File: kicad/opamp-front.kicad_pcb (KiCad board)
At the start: 2 copper layers, 101.3 x 102.4 mm, 91 parts, among them J1 INPUT, J2 GND, J3 SPK, J4 GND, J5 B+, J6 B-, Q1 BD140, Q10 BD139, Q11 BD139, Q12 BD140, Q13 MJL1302C, Q2 2N3906, Q3 2N5551, Q4 2N5401, Q5 2N5551, Q6 2N5401, Q7 BD139, Q8 2N3904, Q9 MJL3281C, U1 LM4562

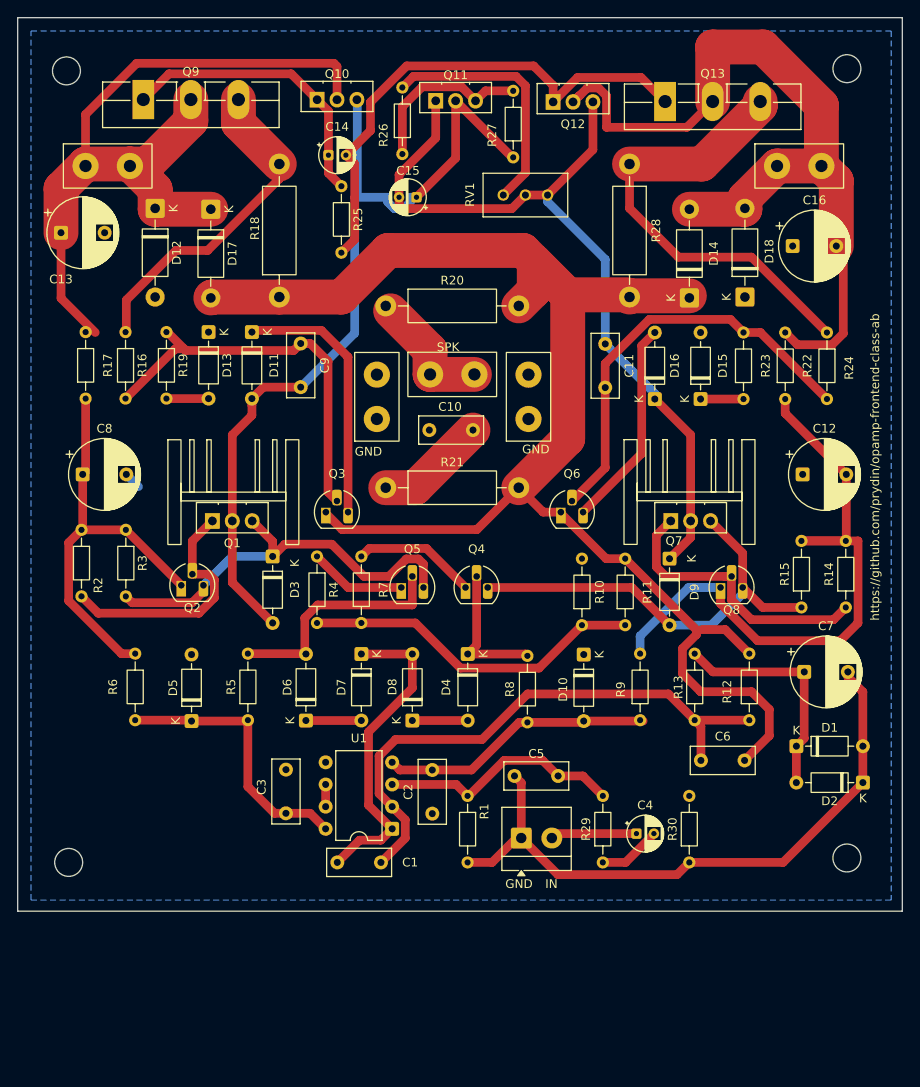
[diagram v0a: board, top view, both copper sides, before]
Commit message: WIP
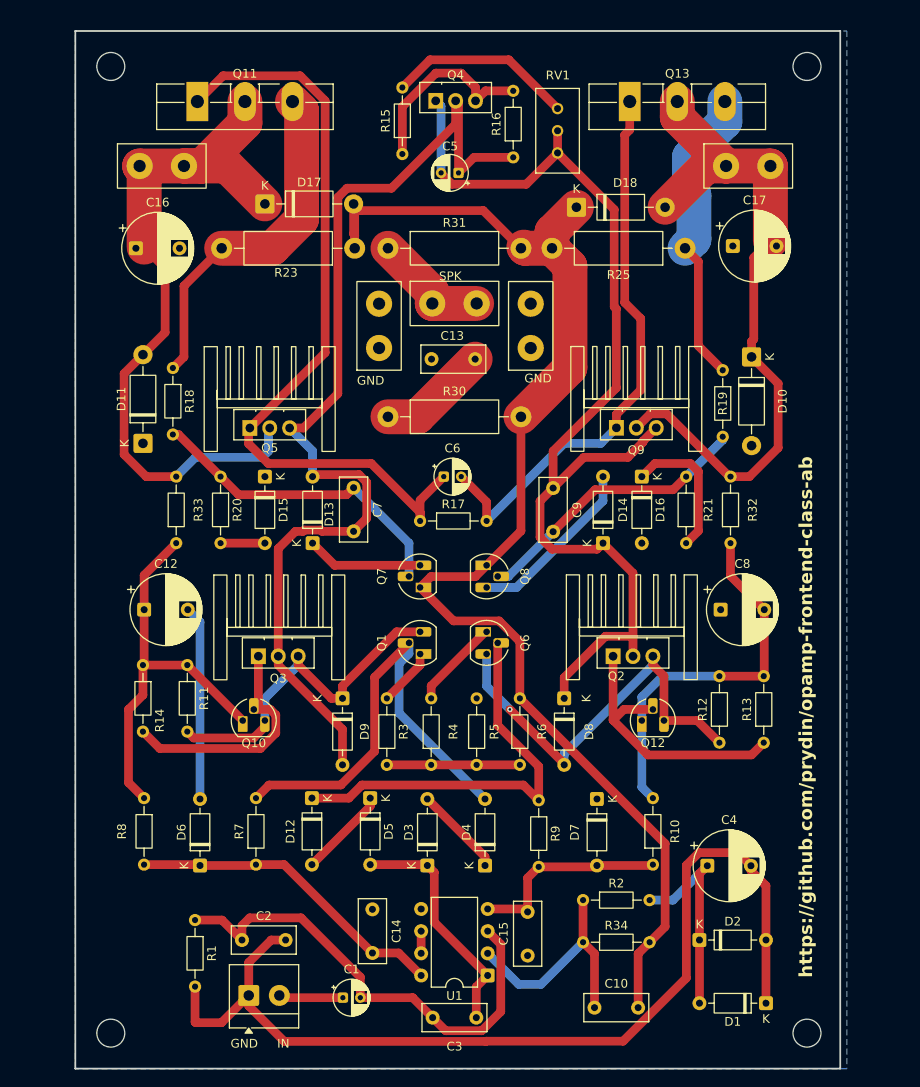
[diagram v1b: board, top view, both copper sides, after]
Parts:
- removed the Q10 at (85.1, 41.9)
- removed R29: 470, Resistor_THT:R_Axial_DIN0204_L3.6mm_D1.6mm_P7.62mm_Horizontal
- removed the R30 at (127.7, 129.3)
- added Q5: BD139, Package_TO_SOT_THT:TO-126-3_Vertical, F.Cu at (77.4, 79.5)
- added REF**: Heatsink, Custom:Heatsink, F.Cu at (79.7, 75.2)
- added REF**: Heatsink, Custom:Heatsink, F.Cu at (121.7, 75.2)
- Q10: renamed from Q2; value 2N3906 -> 2N2906
- Q12: renamed from Q8; value 2N3904 -> 2N2904
- moved C2 40.8 mm to (76.5, 138.2), turned to 0 degrees
- moved R17 39.4 mm to (96.9, 90.2), turned to 0 degrees
- moved C6 39.1 mm to (99.6, 85.1)
- moved C1 38.5 mm to (88.1, 144.8)
- moved Q9 38.0 mm to (119.4, 79.5)
- moved J3 36.1 mm to (77.3, 144.5)
- moved R1 34.3 mm to (71.1, 135.9)
- moved R34 31.8 mm to (115.6, 138.4), turned to 0 degrees
- moved C10 30.8 mm to (116.9, 145.9)
- moved D1 27.6 mm to (136.5, 145.4)
- moved D11 27.0 mm to (65.2, 81.3), turned to 90 degrees
- moved D4 26.4 mm to (104.3, 129.6)
- moved D3 25.4 mm to (97.7, 129.6), turned to 90 degrees
- moved D13 25.2 mm to (84.6, 92.7), turned to 90 degrees
- moved C4 24.8 mm to (129.8, 129.7)
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- renumbered C4 to C1, C6 to C10, C8 to C12, C10 to C13, C3 to C14, C2 to C15, C13 to C16, C16 to C17, C5 to C2, C1 to C3, C7 to C4, C15 to C5, C14 to C6, C9 to C7, C12 to C8, C11 to C9, D2 to D1, D18 to D10, D12 to D11, D4 to D12, D11 to D13, D16 to D14, D13 to D15, D15 to D16, D14 to D18, D1 to D2, D7 to D3, D6 to D4, D8 to D5, D5 to D6, D10 to D7, D9 to D8, D3 to D9, J5 to J1, J3 to J2, J1 to J3, J6 to J5, J2 to J6, Q5 to Q1, Q9 to Q11, Q7 to Q2, Q1 to Q3, Q11 to Q4, Q4 to Q6, Q3 to Q7, Q6 to Q8, Q12 to Q9, R9 to R10, R3 to R11, R15 to R12, R14 to R13, R2 to R14, R26 to R15, R27 to R16, R25 to R17, R16 to R18, R24 to R19, R13 to R2, R19 to R20, R23 to R21, R18 to R23, R28 to R25, R4 to R3, R21 to R30, R20 to R31, R22 to R32, R17 to R33, R12 to R34, R7 to R4, R10 to R5, R11 to R6, R5 to R7, R6 to R8, R8 to R9
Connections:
- C1 pad 2: Net-(C4-Pad2) -> Net-(U1A-+)
- C3 pad 1: Net-(U1A--) -> Net-(U1A-+)
- D10 pad 1: GND -> /B-
- D10 pad 2: /B- -> GND
- D11 pad 1: /B+ -> GND
- D11 pad 2: GND -> /B+
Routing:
- net Net-(Q11-B): track 33.4 -> 90.1 mm
- net GNDA: track 72.8 -> 114.6 mm
- net Net-(U1A--): track 66.1 -> 27.3 mm
- net Net-(D14-K): track 93.8 -> 126.2 mm
- net Net-(D12-K): track 16.2 -> 47.3 mm
- net Net-(Q12-E): track 73.8 -> 43.8 mm
- net Net-(U1A-+): track 27.9 -> 55.5 mm
- net Net-(D4-A): track 27.1 -> 52.3 mm
- net Net-(R3-Pad2): track 39.5 -> 15.2 mm
- net Net-(D17-A): track 177.5 -> 154.4 mm
- net Net-(D13-A): track 101.1 -> 121.6 mm
- net GND: track 1.98 -> 22.3 mm
- net /B-: track 96.2 -> 78.3 mm
- net Net-(Q13-E): track 51.8 -> 34.9 mm
- net Net-(D13-K): track 29.8 -> 13.4 mm
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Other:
- board size 101.3 x 102.4 mm -> 87.6 x 118.9 mm

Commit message: Restored after rebase mishap
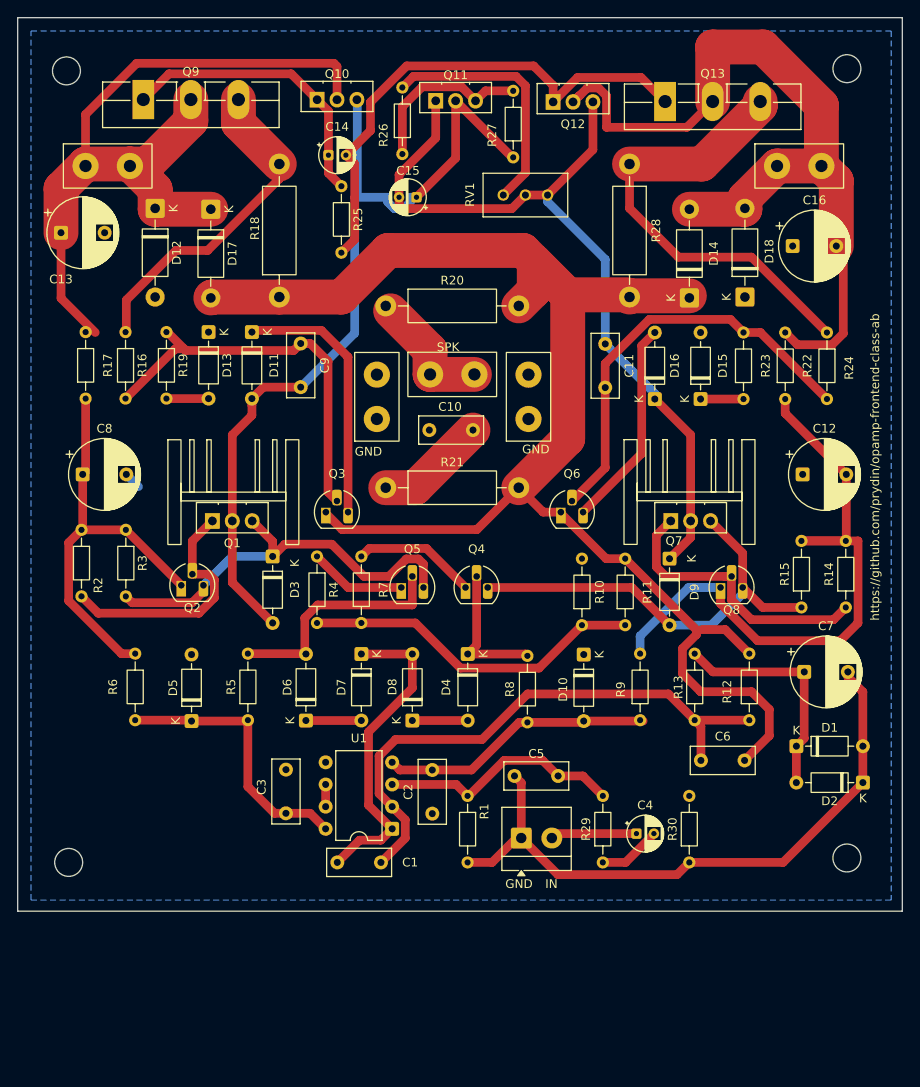
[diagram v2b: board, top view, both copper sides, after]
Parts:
- removed the Q5 at (77.4, 79.5)
- removed the REF** at (79.7, 75.2)
- removed the REF** at (121.7, 75.2)
- added Q10: BD139, Package_TO_SOT_THT:TO-126-3_Vertical, F.Cu at (85.1, 41.9)
- added R29: 470, Resistor_THT:R_Axial_DIN0204_L3.6mm_D1.6mm_P7.62mm_Horizontal, F.Cu at (117.8, 129.3)
- added R30: 10, Resistor_THT:R_Axial_DIN0204_L3.6mm_D1.6mm_P7.62mm_Horizontal, F.Cu at (127.7, 129.3)
- Q2: renamed from Q10; value 2N2906 -> 2N3906
- Q8: renamed from Q12; value 2N2904 -> 2N3904
- moved C5 40.8 mm to (112.7, 119.4), turned to 180 degrees
- moved R25 39.4 mm to (87.9, 51.8), turned to -90 degrees
- moved C14 39.1 mm to (86.4, 48.3)
- moved C4 38.5 mm to (121.7, 126.0)
- moved Q12 38.0 mm to (112.1, 42.2)
- moved J1 36.1 mm to (108.5, 126.5)
- moved R1 34.3 mm to (102.3, 121.7)
- moved R12 31.8 mm to (134.6, 113.0), turned to 90 degrees
- moved C6 30.8 mm to (129.1, 117.6)
- moved D2 27.6 mm to (147.6, 120.1)
- moved D12 27.0 mm to (66.5, 54.4), turned to -90 degrees
- moved D6 26.4 mm to (83.8, 113.0)
- moved D7 25.4 mm to (90.2, 105.4), turned to -90 degrees
- moved D11 25.2 mm to (77.6, 68.5), turned to -90 degrees
- moved C7 24.8 mm to (140.9, 107.5)
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- renumbered C3 to C1, C13 to C10, C9 to C11, C8 to C12, C16 to C13, C6 to C14, C5 to C15, C17 to C16, C15 to C2, C14 to C3, C1 to C4, C2 to C5, C10 to C6, C4 to C7, C12 to C8, C7 to C9, D2 to D1, D7 to D10, D13 to D11, D11 to D12, D15 to D13, D18 to D14, D16 to D15, D14 to D16, D10 to D18, D1 to D2, D9 to D3, D12 to D4, D6 to D5, D4 to D6, D3 to D7, D5 to D8, D8 to D9, J3 to J1, J6 to J2, J2 to J3, J1 to J5, J5 to J6, Q3 to Q1, Q4 to Q11, Q9 to Q12, Q7 to Q3, Q6 to Q4, Q1 to Q5, Q8 to Q6, Q2 to Q7, Q11 to Q9, R5 to R10, R6 to R11, R34 to R12, R2 to R13, R13 to R14, R12 to R15, R18 to R16, R33 to R17, R23 to R18, R20 to R19, R14 to R2, R31 to R20, R30 to R21, R32 to R22, R21 to R23, R19 to R24, R17 to R25, R15 to R26, R16 to R27, R25 to R28, R11 to R3, R3 to R4, R7 to R5, R8 to R6, R4 to R7, R9 to R8, R10 to R9
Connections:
- C1 pad 1: Net-(U1A-+) -> Net-(U1A--)
- C4 pad 2: Net-(U1A-+) -> Net-(C4-Pad2)
- D12 pad 1: GND -> /B+
- D12 pad 2: /B+ -> GND
- D18 pad 1: /B- -> GND
- D18 pad 2: GND -> /B-
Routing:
- net Net-(Q10-E): track 90.1 -> 33.4 mm
- net GNDA: track 114.6 -> 72.8 mm
- net Net-(U1A--): track 27.3 -> 66.1 mm
- net Net-(D16-K): track 126.2 -> 93.8 mm
- net Net-(D4-K): track 47.3 -> 16.2 mm
- net Net-(Q8-E): track 43.8 -> 73.8 mm
- net Net-(U1A-+): track 55.5 -> 27.9 mm
- net Net-(D6-A): track 52.3 -> 27.1 mm
- net Net-(R10-Pad1): track 15.2 -> 39.5 mm
- net Net-(D14-K): track 154.4 -> 177.5 mm
- net Net-(D11-A): track 121.6 -> 101.1 mm
- net GND: track 22.3 -> 1.98 mm
- net /B-: track 78.3 -> 96.2 mm
- net Net-(Q13-E): track 34.9 -> 51.8 mm
- net Net-(D11-K): track 13.4 -> 29.8 mm
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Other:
- board size 87.6 x 118.9 mm -> 101.3 x 102.4 mm
